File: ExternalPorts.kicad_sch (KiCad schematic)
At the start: 13 parts, among them J10 Conn_01x04, J11 Conn_01x06, J12 Conn_01x06, J13 Conn_01x04, J14 Conn_01x04, J15 Conn_01x04, J16 Conn_01x03, J17 Conn_01x06, J5 Conn_01x06, J6 Conn_01x06, J7 Conn_01x06, J8 Conn_01x04, J9 Conn_01x04

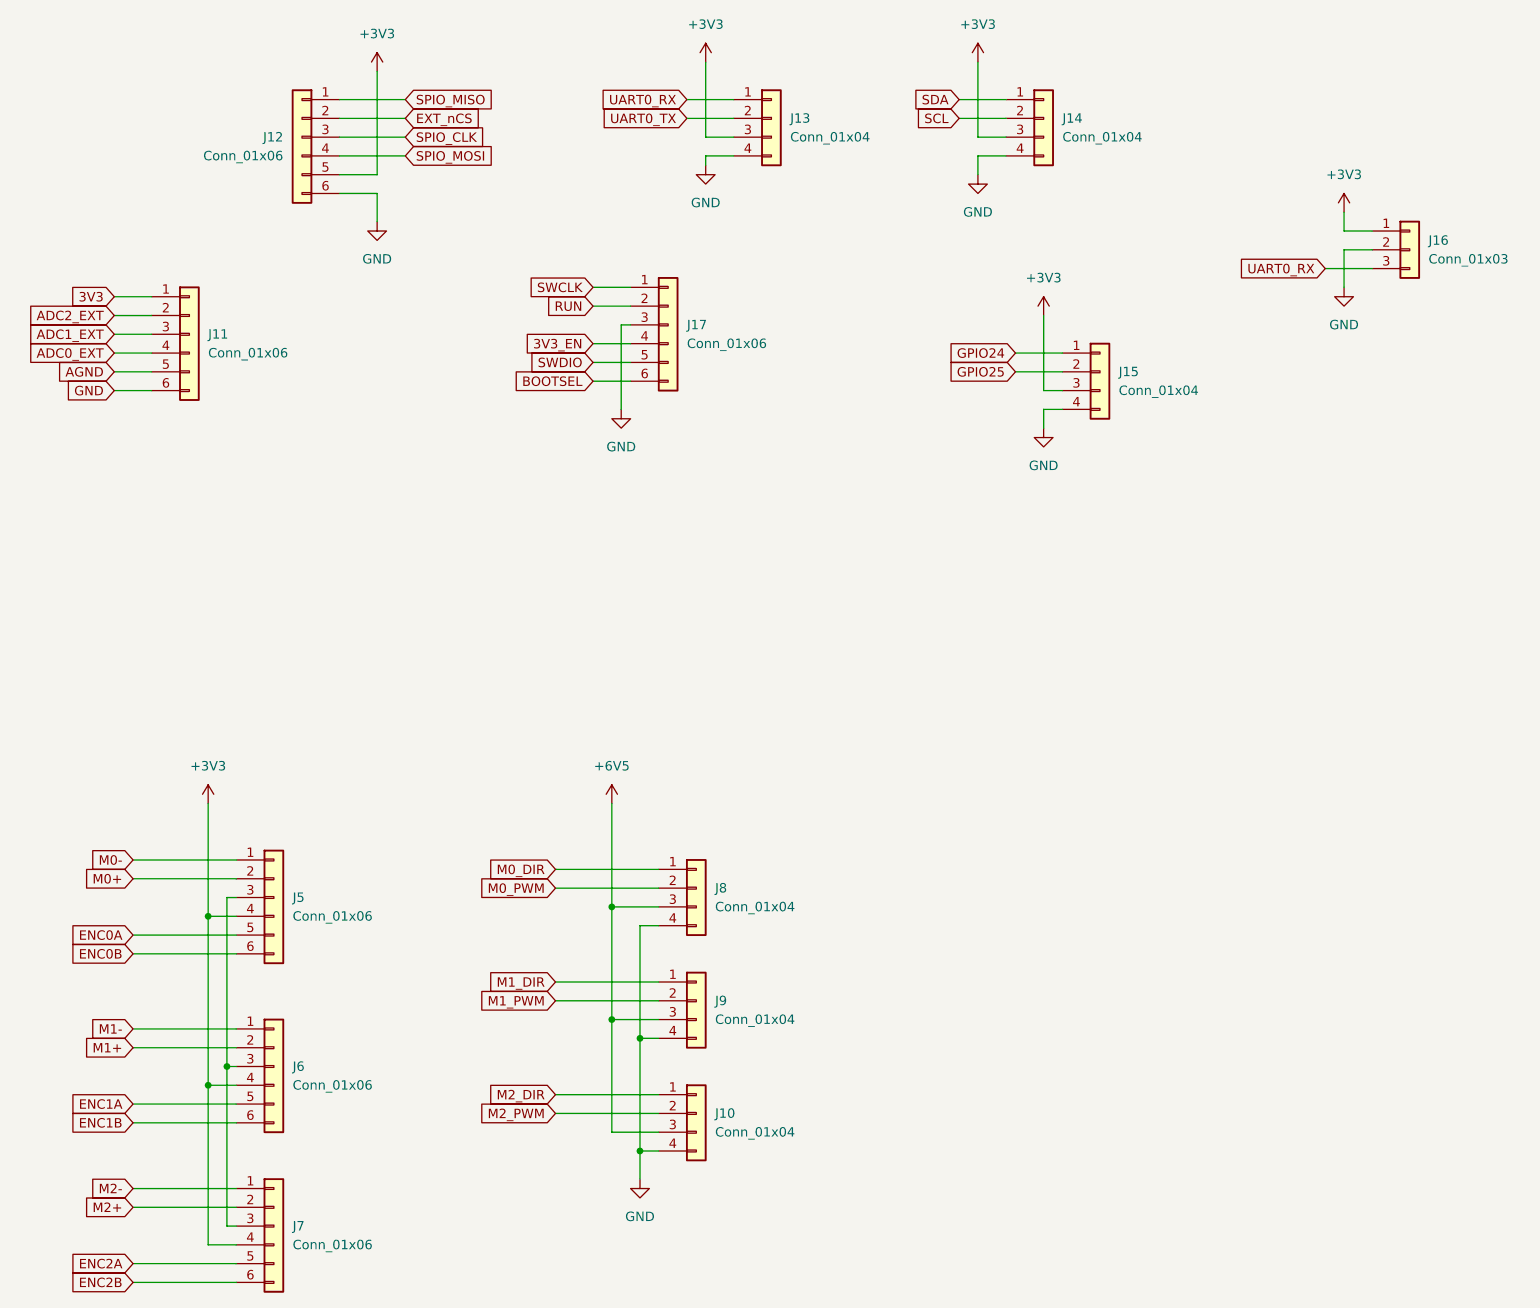
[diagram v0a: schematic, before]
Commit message: Add files via upload
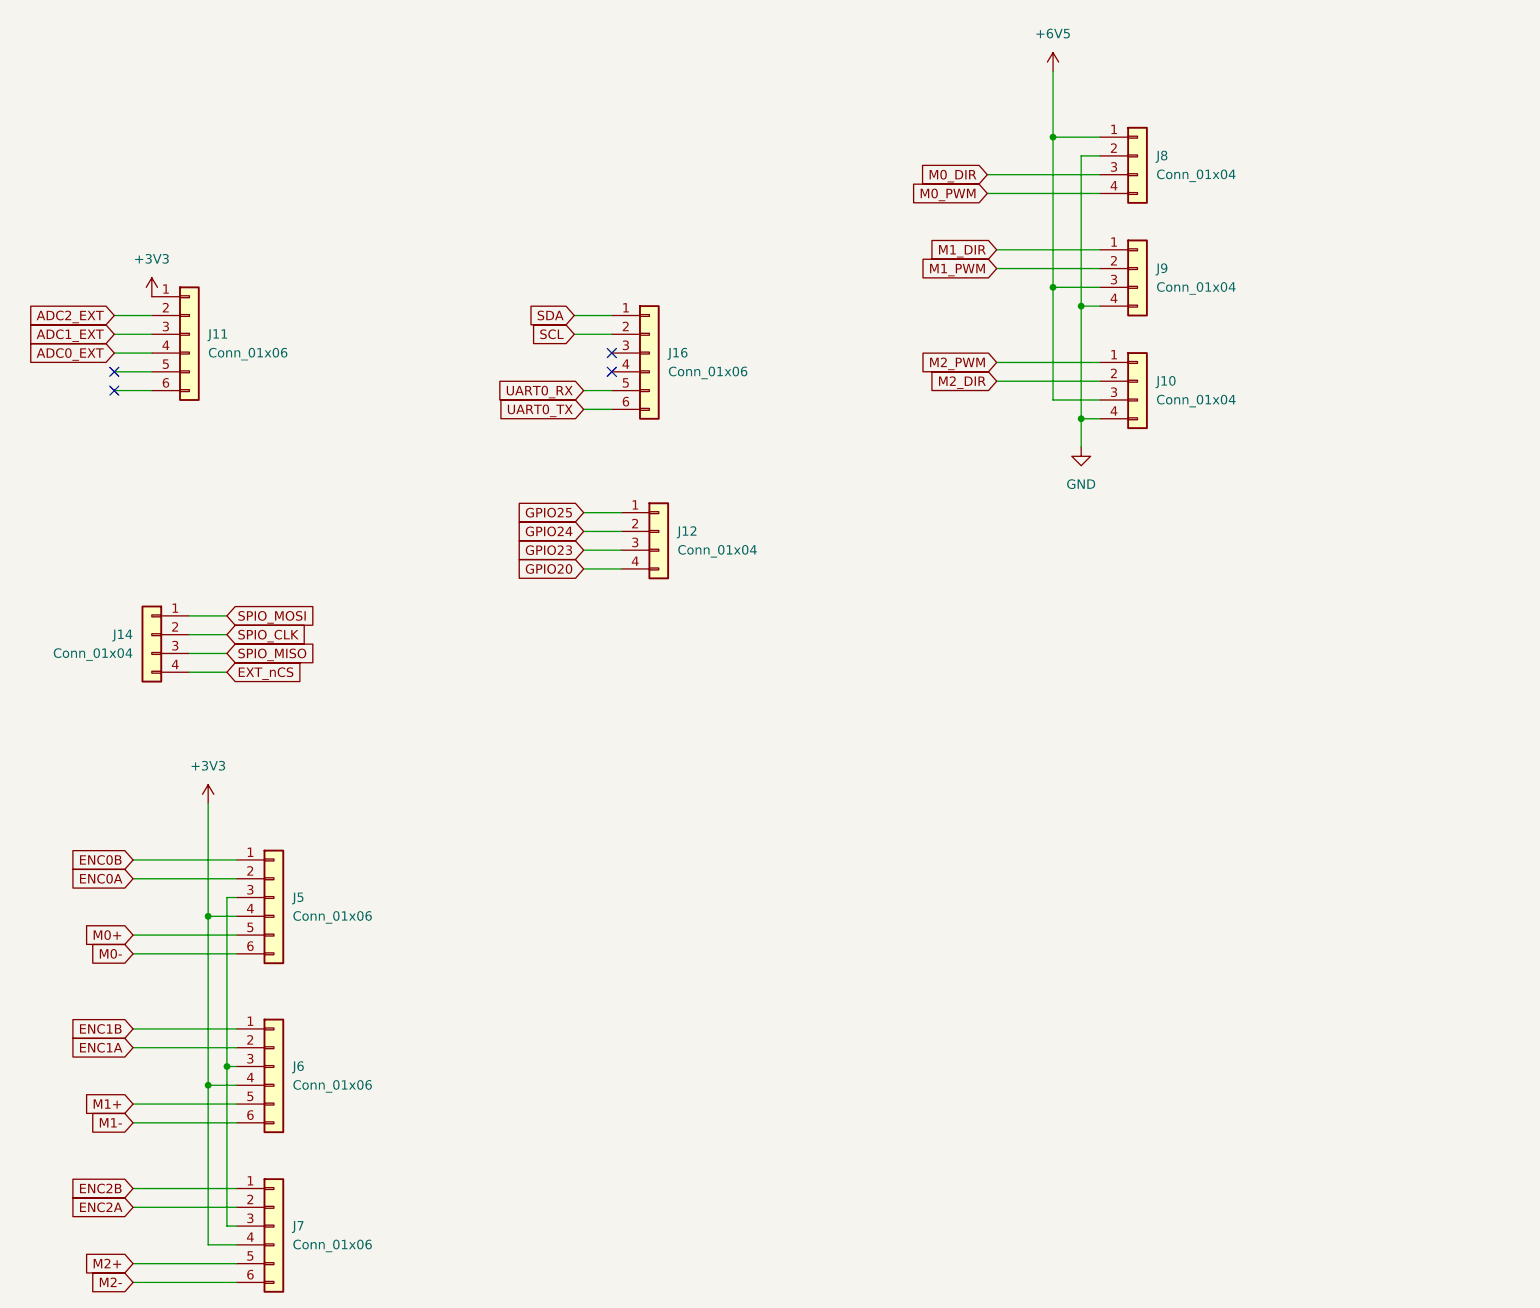
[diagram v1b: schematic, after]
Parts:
- removed J12, J17: Conn_01x06, Connector_JST:JST_PH_B6B-PH-K_1x06_P2.00mm_Vertical, symbol Connector_Generic:Conn_01x06
- removed J13, J15: Conn_01x04, Connector_Hirose:Hirose_DF63M-4P-3.96DSA_1x04_P3.96mm_Vertical, symbol Connector_Generic:Conn_01x04
- removed J16: Conn_01x03, Connector:FanPinHeader_1x03_P2.54mm_Vertical, symbol Connector_Generic:Conn_01x03
- added J12: Conn_01x04, Connector_Hirose:Hirose_DF13-04P-1.25DSA_1x04_P1.25mm_Vertical, symbol Connector_Generic:Conn_01x04
- added J16: Conn_01x06, Connector_Hirose:Hirose_DF13-06P-1.25DSA_1x06_P1.25mm_Vertical, symbol Connector_Generic:Conn_01x06
- J10, J14, J8, J9: footprint Connector_Hirose:Hirose_DF63M-4P-3.96DSA_1x04_P3.96mm_Vertical -> Connector_Hirose:Hirose_DF13-04P-1.25DSA_1x04_P1.25mm_Vertical
- J11, J5, J6, J7: footprint Connector_JST:JST_PH_B6B-PH-K_1x06_P2.00mm_Vertical -> Connector_Hirose:Hirose_DF13-06P-1.25DSA_1x06_P1.25mm_Vertical
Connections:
- net 3V3 is gone; now on net +3V3: J11.1 (Pin_1)
- net +3V3: no longer J14.3 (Pin_3)
- net +6V5: now also J8.1 (Pin_1); no longer J8.3 (Pin_3)
- net ENC0A: now also J5.2 (Pin_2); no longer J5.5 (Pin_5)
- net ENC0B: now also J5.1 (Pin_1); no longer J5.6 (Pin_6)
- net ENC1A: now also J6.2 (Pin_2); no longer J6.5 (Pin_5)
- net ENC1B: now also J6.1 (Pin_1); no longer J6.6 (Pin_6)
- net ENC2A: now also J7.2 (Pin_2); no longer J7.5 (Pin_5)
- net ENC2B: now also J7.1 (Pin_1); no longer J7.6 (Pin_6)
- net EXT_nCS: now also J14.4 (Pin_4)
- net GND: now also J8.2 (Pin_2); no longer J11.6 (Pin_6), J14.4 (Pin_4), J8.4 (Pin_4)
- net GPIO24: now also J12.2 (Pin_2)
- net GPIO25: now also J12.1 (Pin_1)
- net M0+: now also J5.5 (Pin_5); no longer J5.2 (Pin_2)
- net M0-: now also J5.6 (Pin_6); no longer J5.1 (Pin_1)
- net M0_DIR: now also J8.3 (Pin_3); no longer J8.1 (Pin_1)
- net M0_PWM: now also J8.4 (Pin_4); no longer J8.2 (Pin_2)
- net M1+: now also J6.5 (Pin_5); no longer J6.2 (Pin_2)
- net M1-: now also J6.6 (Pin_6); no longer J6.1 (Pin_1)
- net M2+: now also J7.5 (Pin_5); no longer J7.2 (Pin_2)
- net M2-: now also J7.6 (Pin_6); no longer J7.1 (Pin_1)
- net M2_DIR: now also J10.2 (Pin_2); no longer J10.1 (Pin_1)
- net M2_PWM: now also J10.1 (Pin_1); no longer J10.2 (Pin_2)
- net SCL: now also J16.2 (Pin_2); no longer J14.2 (Pin_2)
- net SDA: now also J16.1 (Pin_1); no longer J14.1 (Pin_1)
- net SPIO_CLK: now also J14.2 (Pin_2)
- net SPIO_MISO: now also J14.3 (Pin_3)
- net SPIO_MOSI: now also J14.1 (Pin_1)
- net UART0_RX: now also J16.5 (Pin_5)
- net UART0_TX: now also J16.6 (Pin_6)
- net AGND: no longer names the net of J11.5 (Pin_5)
- new net GPIO20: J12.4 (Pin_4)
- new net GPIO23: J12.3 (Pin_3)
- no-connect marks 0 -> 4
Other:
- moved on the sheet: J10, J8, J9
